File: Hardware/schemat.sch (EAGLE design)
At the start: 25 parts, among them IC1 MEGA32-A, IC2 7805DT, J1 12v, J2 PIN1-2, J3 PIN1-2, T1 BC237

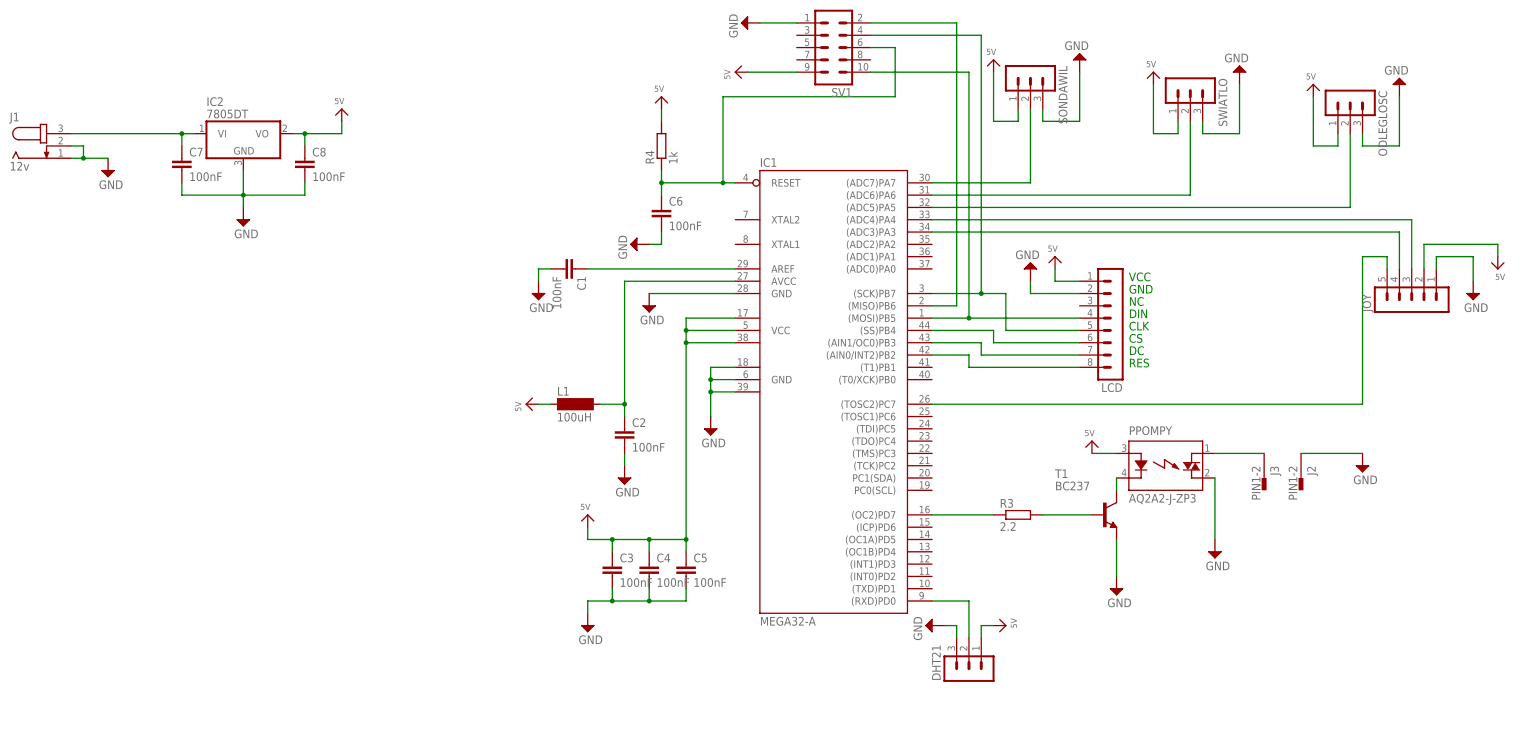
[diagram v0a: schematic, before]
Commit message: dokumentacja
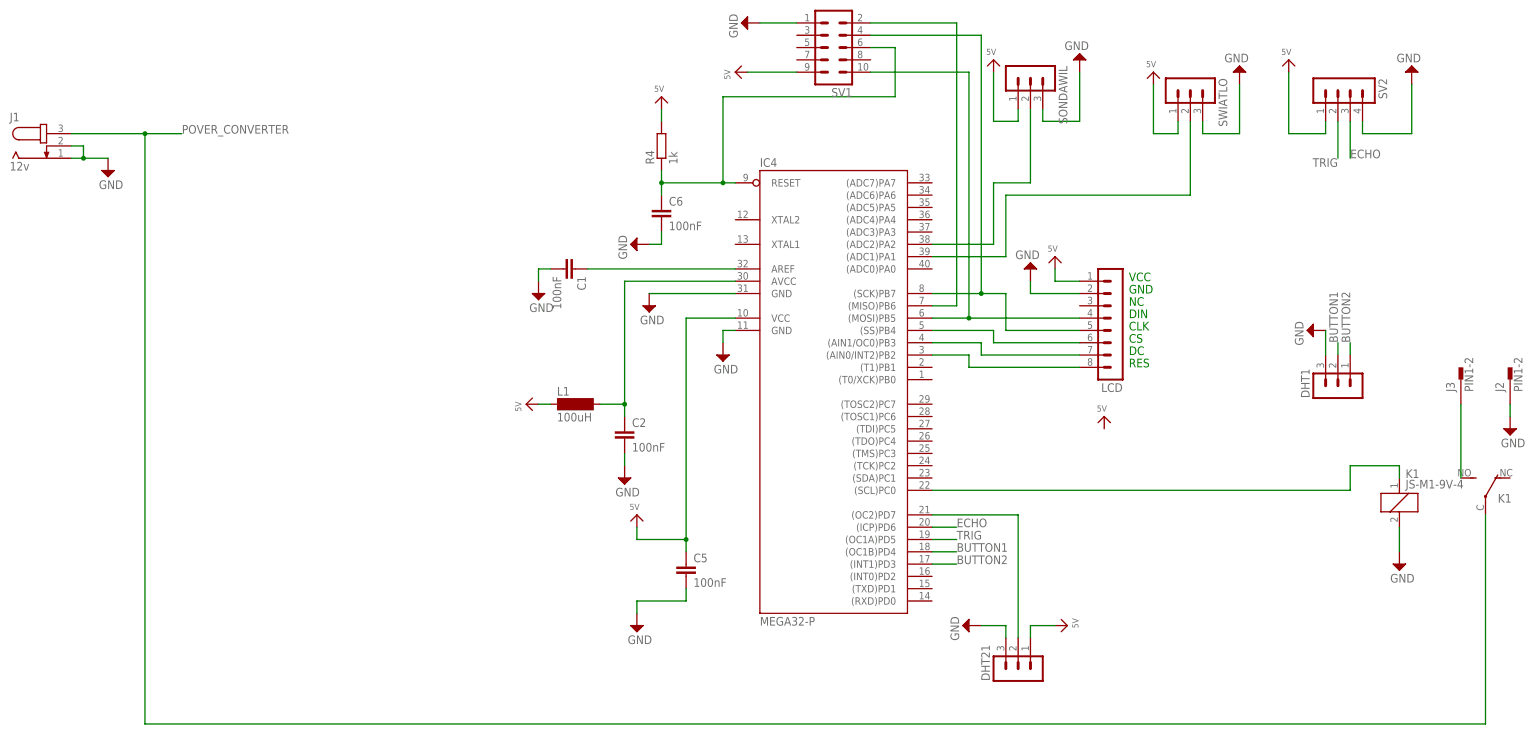
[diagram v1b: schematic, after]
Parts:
- removed C3, C4, C7, C8: 100nF, capacitor-wima:C2.5/6
- removed IC1: MEGA32-A, atmel:MEGA32-A
- removed IC2: 7805DT, linear:7805DT
- removed JOY: (no value), con-lstb:MA05-1
- removed ODLEGLOSC: (no value), con-lstb:MA03-1
- removed PPOMPY: AQ2A2-J-ZP3, relay:AQ2A2-J-ZP3
- removed R3: 2.2, rcl:R-EU_0207/15
- removed T1: BC237, transistor:BC237
- added DHT1: (no value), con-lstb:MA03-1
- added IC4: MEGA32-P, atmel:MEGA32-P
- added K1: JS-M1-9V-4, relay:JS-M1-9V-4
- added SV2: (no value), con-lstb:MA04-1
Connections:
- removed net N$14: IC1.(OC2)PD7, R3.1
- removed net N$15: R3.2, T1.B
- removed net N$16: IC1.(TOSC2)PC7, JOY.5
- removed net N$17: IC1.(ADC3)PA3, JOY.4
- removed net N$18: IC1.(ADC4)PA4, JOY.3
- removed net N$19: PPOMPY.K, T1.C
- removed net N$22: J3.1, PPOMPY.DS1
- removed net N$24: C7.1, IC2.VI, J1.3
- new net BUTTON1: DHT1.2, IC4.(OC1B)PD4
- new net BUTTON2: DHT1.1, IC4.(INT1)PD3
- new net ECHO: SV2.3
- new net N$1: IC4.(ADC1)PA1, SWIATLO.2
- new net POVER_CONVERTER: J1.3, K12.P
- new net TRIG: SV2.2
- net GND: now also DHT1.3, IC4.GND, IC4.GND@1, K11.2, SV2.4; no longer C3.2, C4.2, C7.2, C8.2, IC1.GND, IC1.GND1, IC1.GND2, IC1.GND@1, IC2.GND, JOY.1, ODLEGLOSC.3, PPOMPY.DS2, T1.E
- net N$10: now also IC4.(OC2)PD7; no longer IC1.(RXD)PD0
- net N$11: now also J3.1, K12.S; no longer IC1.(ADC5)PA5, ODLEGLOSC.2
- net N$12: now also IC4.(ADC2)PA2; no longer IC1.(ADC7)PA7
- net N$13: now also IC4.(SCL)PC0, K11.1; no longer IC1.(ADC6)PA6, SWIATLO.2
- net N$2: now also IC4.RESET; no longer IC1.RESET
- net N$20: now also IC4.(MISO)PB6; no longer IC1.(MISO)PB6
- net N$3: now also IC4.(MOSI)PB5; no longer IC1.(MOSI)PB5
- net N$4: now also IC4.AREF; no longer IC1.AREF
- net N$5: now also IC4.AVCC; no longer IC1.AVCC
- net N$6: now also IC4.(SCK)PB7; no longer IC1.(SCK)PB7
- net N$7: now also IC4.(SS)PB4; no longer IC1.(SS)PB4
- net N$8: now also IC4.(AIN1/OC0)PB3; no longer IC1.(AIN1/OC0)PB3
- net N$9: now also IC4.(AIN0/INT2)PB2; no longer IC1.(AIN0/INT2)PB2
- net VCC: now also IC4.VCC, SV2.1; no longer C3.1, C4.1, C8.1, IC1.VCC, IC1.VCC1, IC1.VCC2, IC2.VO, JOY.2, ODLEGLOSC.1, PPOMPY.A
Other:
- moved on the sheet: DHT21, J2, J3
